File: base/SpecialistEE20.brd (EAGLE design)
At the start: 55.9 x 6.6 mm, 109 parts, among them X1 SCART-F

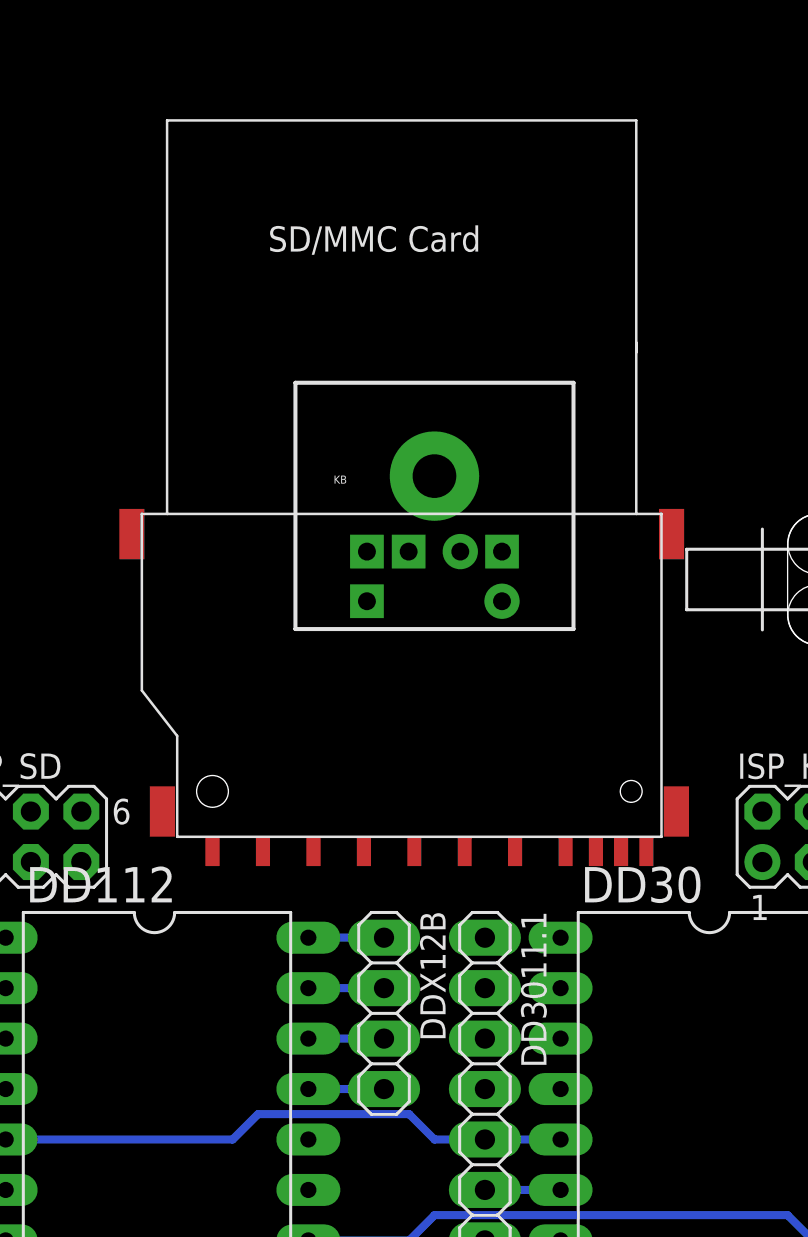
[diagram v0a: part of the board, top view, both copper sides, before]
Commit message: .
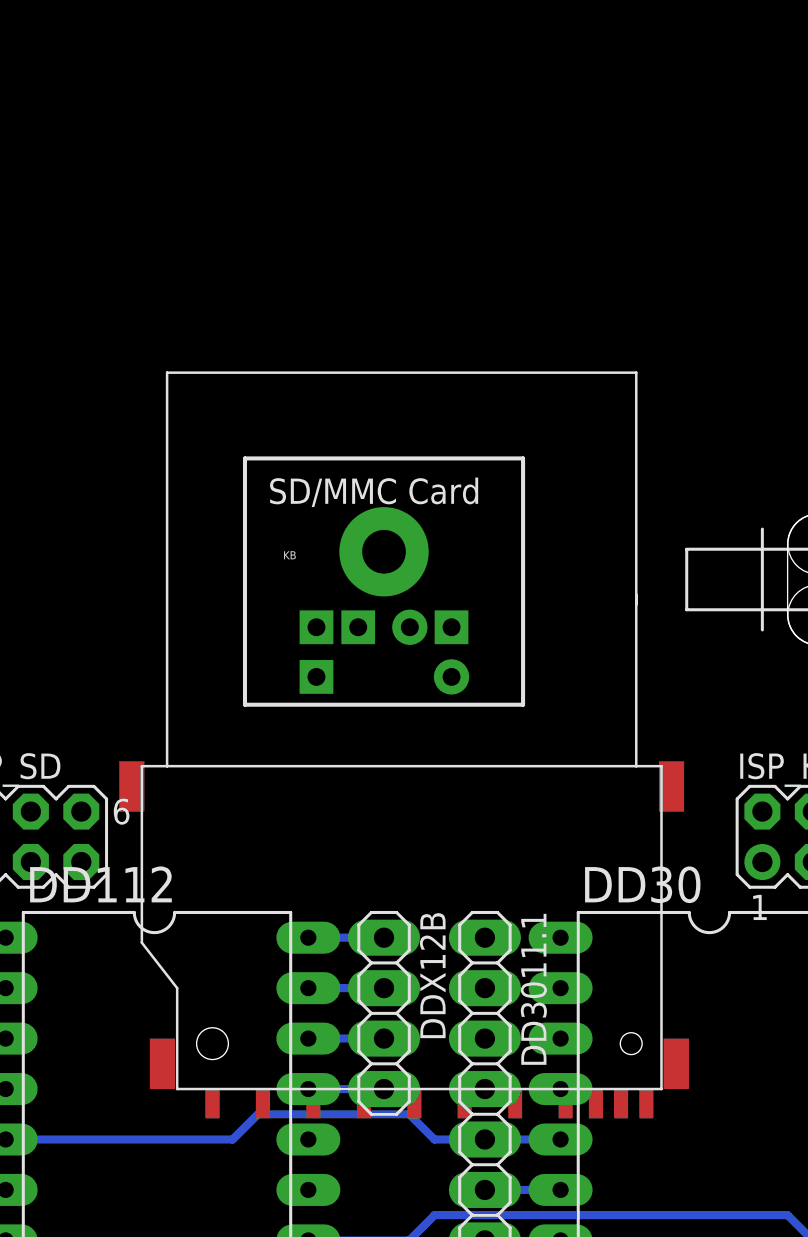
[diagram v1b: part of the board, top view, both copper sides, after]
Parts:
- moved J1 12.7 mm to (59.7, 165.1)
- moved KB 4.58 mm to (58.4, 184.2)
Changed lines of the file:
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@@
 <board>
 <plain>
-<dimension x1="191.77" y1="199.39" x2="24.13" y2="208.28" x3="107.95" y3="54.61" textsize="1.778" layer="21" dtype="horizontal"/>
-<dimension x1="15.24" y1="73.66" x2="19.05" y2="189.23" x3="243.84" y3="131.445" textsize="1.778" layer="21" dtype="vertical"/>
+<dimension x1="190.5" y1="207.01" x2="19.05" y2="199.39" x3="104.775" y3="54.61" textsize="1.778" layer="21" dtype="horizontal"/>
+<dimension x1="15.24" y1="73.66" x2="12.7" y2="185.42" x3="228.6" y3="129.54" textsize="1.778" layer="21" dtype="vertical"/>
 <text x="248.92" y="93.98" size="6.4516" layer="22" rot="R180">21x13</text>
 <text x="228.6" y="121.92" size="6.4516" layer="22">220х135 вост экс нов</text>
@@
 <element name="DD3011.1" library="Разъёмы штырьковые 2.54мм" package="1X20" value="" x="63.5" y="135.89" rot="R270"/>
 <element name="DD3011.2" library="Разъёмы штырьковые 2.54мм" package="1X20" value="" x="86.36" y="135.89" rot="R270"/>
-<element name="KB" library="Speccy" package="MINI-DIN6" value="MINI-DIN6" x="60.96" y="187.96"/>
+<element name="KB" library="Speccy" package="MINI-DIN6" value="MINI-DIN6" x="58.42" y="184.15"/>
 <element name="DD45" library="74xx-eu" package="DIL14" value="К555ИЕ19" x="203.2" y="105.41"/>
 <element name="R105" library="rcl" package="M0805" value="4k7" x="208.28" y="-5.08" rot="MR0"/>
@@
 <attribute name="OC_FARNELL" value="unknown" x="106.68" y="176.53" size="1.778" layer="27" rot="R180" display="off"/>
 </element>
-<element name="J1" library="Speccy" package="SDCMF-10915W010" value="" x="59.69" y="177.8" rot="R180"/>
+<element name="J1" library="Speccy" package="SDCMF-10915W010" value="" x="59.69" y="165.1" rot="R180"/>
 <element name="U$2" library="ESR_NM8032" package="SWITCH9X4" value="SWITCH9X4" x="-12.7" y="152.4"/>
 <element name="R13" library="rcl" package="M1206" value="2k" x="190.5" y="184.15" rot="R180"/>
@@
 <wire x1="102.87" y1="152.4" x2="105.41" y2="163.83" width="0" layer="19" extent="1-1"/>
 <wire x1="82.55" y1="166.37" x2="105.41" y2="163.83" width="0" layer="19" extent="1-1"/>
-<wire x1="73.136125" y1="166.37" x2="82.55" y2="166.37" width="0" layer="19" extent="1-1"/>
-<wire x1="72.898" y1="180.34" x2="73.136125" y2="166.37" width="0" layer="19" extent="1-1"/>
-<wire x1="64.36" y1="179.46" x2="72.898" y2="180.34" width="0" layer="19" extent="1-1"/>
-<wire x1="45.72" y1="180.34" x2="64.36" y2="179.46" width="0" layer="19" extent="1-1"/>
-<wire x1="47.259875" y1="166.37" x2="45.72" y2="180.34" width="0" layer="19" extent="1-1"/>
-<wire x1="43.18" y1="166.37" x2="47.259875" y2="166.37" width="0" layer="19" extent="1-1"/>
+<wire x1="73.136125" y1="153.67" x2="82.55" y2="166.37" width="0" layer="19" extent="1-1"/>
+<wire x1="72.898" y1="167.64" x2="73.136125" y2="153.67" width="0" layer="19" extent="1-1"/>
+<wire x1="61.82" y1="175.65" x2="72.898" y2="167.64" width="0" layer="19" extent="1-1"/>
+<wire x1="45.72" y1="167.64" x2="61.82" y2="175.65" width="0" layer="19" extent="1-1"/>
+<wire x1="47.259875" y1="153.67" x2="45.72" y2="167.64" width="0" layer="19" extent="1-1"/>
+<wire x1="43.18" y1="166.37" x2="47.259875" y2="153.67" width="0" layer="19" extent="1-1"/>
 <wire x1="24.13" y1="170.18" x2="43.18" y2="166.37" width="0" layer="19" extent="1-1"/>
 <wire x1="20.32" y1="163.83" x2="24.13" y2="170.18" width="0" layer="19" extent="1-1"/>
@@
 <contactref element="ISP_SD" pad="2"/>
 <contactref element="ISP_KB" pad="2"/>
-<wire x1="57.56" y1="179.46" x2="77.47" y2="166.37" width="0" layer="19" extent="1-1"/>
-<wire x1="38.1" y1="166.37" x2="57.56" y2="179.46" width="0" layer="19" extent="1-1"/>
+<wire x1="55.02" y1="175.65" x2="77.47" y2="166.37" width="0" layer="19" extent="1-1"/>
+<wire x1="38.1" y1="166.37" x2="55.02" y2="175.65" width="0" layer="19" extent="1-1"/>
 <wire x1="48.99" y1="136.3726" x2="38.1" y2="166.37" width="0" layer="19" extent="1-1"/>
 <wire x1="48.19" y1="127.7874" x2="48.99" y2="136.3726" width="0" layer="19" extent="1-1"/>
@@
 <contactref element="DD213" pad="1"/>
 <contactref element="R106" pad="1"/>
-<wire x1="79" y1="118.5926" x2="62.26" y2="179.46" width="0" layer="19" extent="1-1"/>
+<wire x1="79" y1="118.5926" x2="59.72" y2="175.65" width="0" layer="19" extent="1-1"/>
 <wire x1="210.5" y1="-6.35" x2="79" y2="118.5926" width="0" layer="19" extent="1-16"/>
 </signal>
@@
 <contactref element="KB" pad="1"/>
 <contactref element="R105" pad="1"/>
-<wire x1="71.9074" y1="116.3" x2="59.66" y2="179.46" width="0" layer="19" extent="1-1"/>
+<wire x1="71.9074" y1="116.3" x2="57.12" y2="175.65" width="0" layer="19" extent="1-1"/>
 <wire x1="209.23" y1="-5.08" x2="71.9074" y2="116.3" width="0" layer="19" extent="1-16"/>
 </signal>
